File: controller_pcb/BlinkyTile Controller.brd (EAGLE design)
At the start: 40 x 25 mm, 31 parts, among them CN1 Battery, CON1 USB_MICROSMT+THRUHULE, Q1 16MHz, T1 SSM3J328R,LF, U1 MK20D--VFM5, U2 W25Q--DVSS(208), U3 74LVC1G17DCK, U4 74LVC1G17DCK, U5 74LVC1G17DCK, U6 TPD4S012

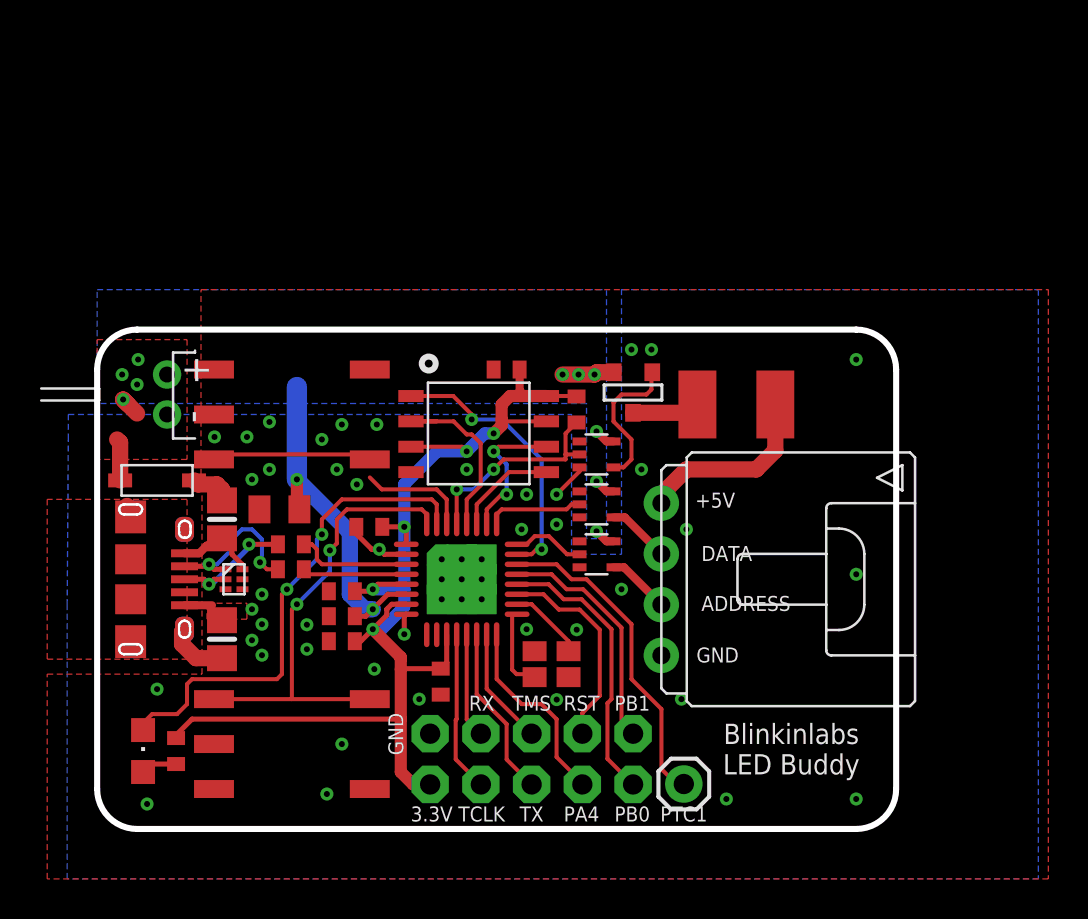
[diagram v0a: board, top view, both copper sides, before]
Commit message: Controller boar design, as released.
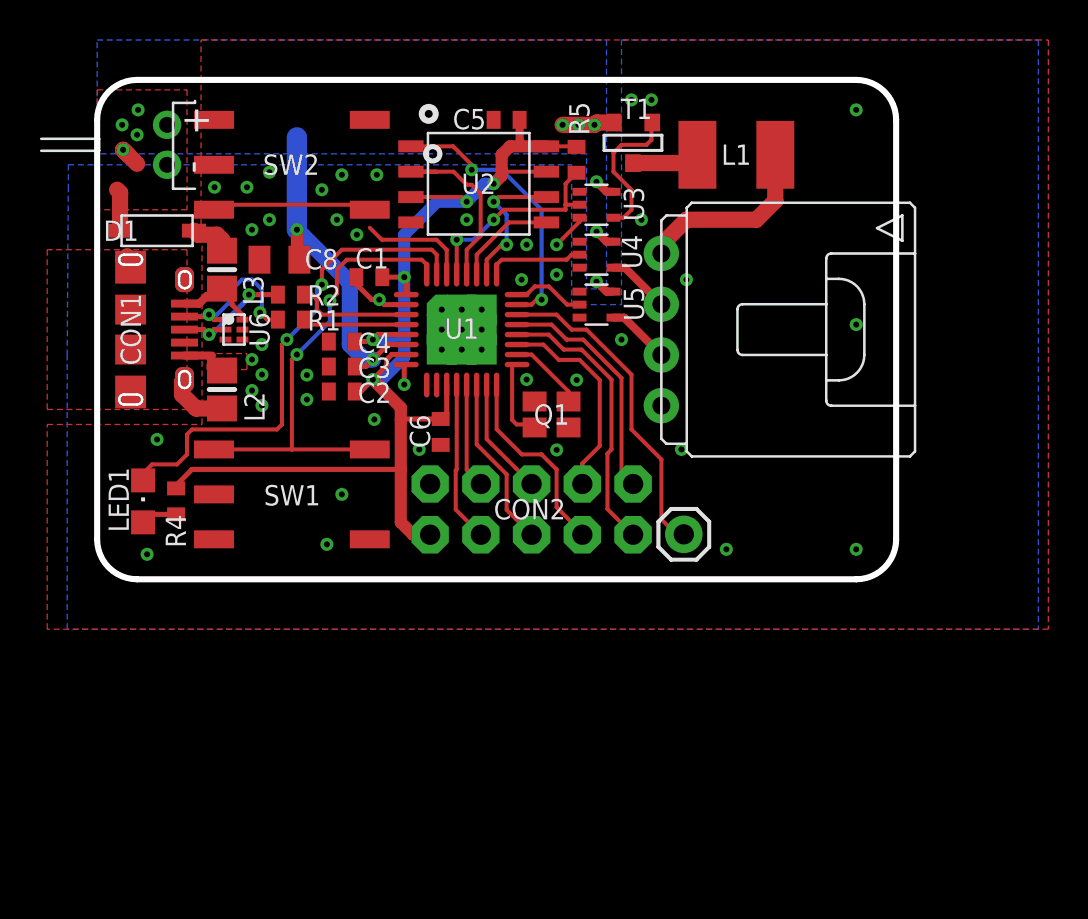
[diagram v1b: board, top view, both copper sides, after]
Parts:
- removed D3: RB161M-20, adafruit:SOD-123
- removed JP1: M05X2NO_SILK, SparkFun-Connectors:2X5_NOSILK
- removed JP3: M01PTH, SparkFun-Connectors:1X01
- removed SV1: LED_OUT, blinkinlabs:DUPONT-4P
- removed U$1: BUTTON_1, blinkinlabs:TD-07XB
- removed U$2: BUTTON_2, blinkinlabs:TD-07XB
- added CON2: M05X2NO_SILK, SparkFun-Connectors:2X5_NOSILK
- added CON3: LED_OUT, blinkinlabs:DUPONT-4P
- added CON4: M01PTH, SparkFun-Connectors:1X01
- added D1: RB161M-20, adafruit:SOD-123
- added SW1: BUTTON_1, blinkinlabs:TD-07XB
- added SW2: BUTTON_2, blinkinlabs:TD-07XB
- R4: value 330 -> 470
- moved T1 12.5 mm to (26.8, 21.9)
- moved C1 12.5 mm to (13.6, 15.1)
- moved C2 12.5 mm to (12.2, 9.40)
- moved C3 12.5 mm to (12.2, 10.7)
- moved C4 12.5 mm to (12.2, 11.9)
- moved C5 12.5 mm to (20.5, 23.0)
- moved C6 12.5 mm to (17.2, 7.38)
- moved C8 12.5 mm to (9.12, 16.0)
- moved CN1 12.5 mm to (3.50, 21.8)
- moved CON1 12.5 mm to (1.68, 12.5)
- moved L1 12.5 mm to (32.0, 21.2)
- moved L2 12.5 mm to (6.25, 9.50)
- moved L3 12.5 mm to (6.25, 15.5)
- moved LED1 12.5 mm to (2.30, 3.90)
- moved Q1 12.5 mm to (22.8, 8.25)
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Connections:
- net +3V3: now also CON2.1; no longer JP1.1
- net +5V: now also D1.C; no longer D3.C
- net ADC15: now also CON4.1; no longer JP3.1
- net BUTTON1: now also SW1.3, SW1.4; no longer U$1.3, U$1.4
- net BUTTON2: now also SW2.1, SW2.2; no longer U$2.1, U$2.2
- net GND: now also CON2.2, CON3.P$4, SW1.1, SW1.2, SW1.5, SW2.3, SW2.4, SW2.5; no longer JP1.2, SV1.P$4, U$1.1, U$1.2, U$1.5, U$2.3, U$2.4, U$2.5
- net LED_DATA: now also CON3.P$2; no longer SV1.P$2
- net N$4: now also CON3.P$3; no longer SV1.P$3
- net N$8: now also CON3.P$1; no longer SV1.P$1
- net N$9: now also D1.A; no longer D3.A
- net PA4: now also CON2.7; no longer JP1.7
- net PB0: now also CON2.9; no longer JP1.9
- net PB1: now also CON2.10; no longer JP1.10
- net RESET: now also CON2.8; no longer JP1.8
- net RX: now also CON2.4; no longer JP1.4
- net TCLK: now also CON2.3; no longer JP1.3
- net TMS: now also CON2.6; no longer JP1.6
- net TX: now also CON2.5; no longer JP1.5
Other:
- board text added: "CON3"
- board text removed: "3.3V"
- board text removed: "Blinkinlabs LED Buddy"
- board text removed: "PA4"
- board text removed: "PB0"
- board text removed: "PB1"
- board text removed: "PTC1"
- board text removed: "RST"
- board text removed: "RX"
- board text removed: "TCLK"
- board text removed: "TMS"
- board text removed: "TX"
